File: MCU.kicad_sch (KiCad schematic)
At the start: 29 parts, among them J3 TAG-Connect, J4 BOOT, J5 USB4110-GF-A, J6 SWD, SW1 1-1571636-0, U15 12MHz, U5 RP2040, U6 W25Q16JVSSIQ

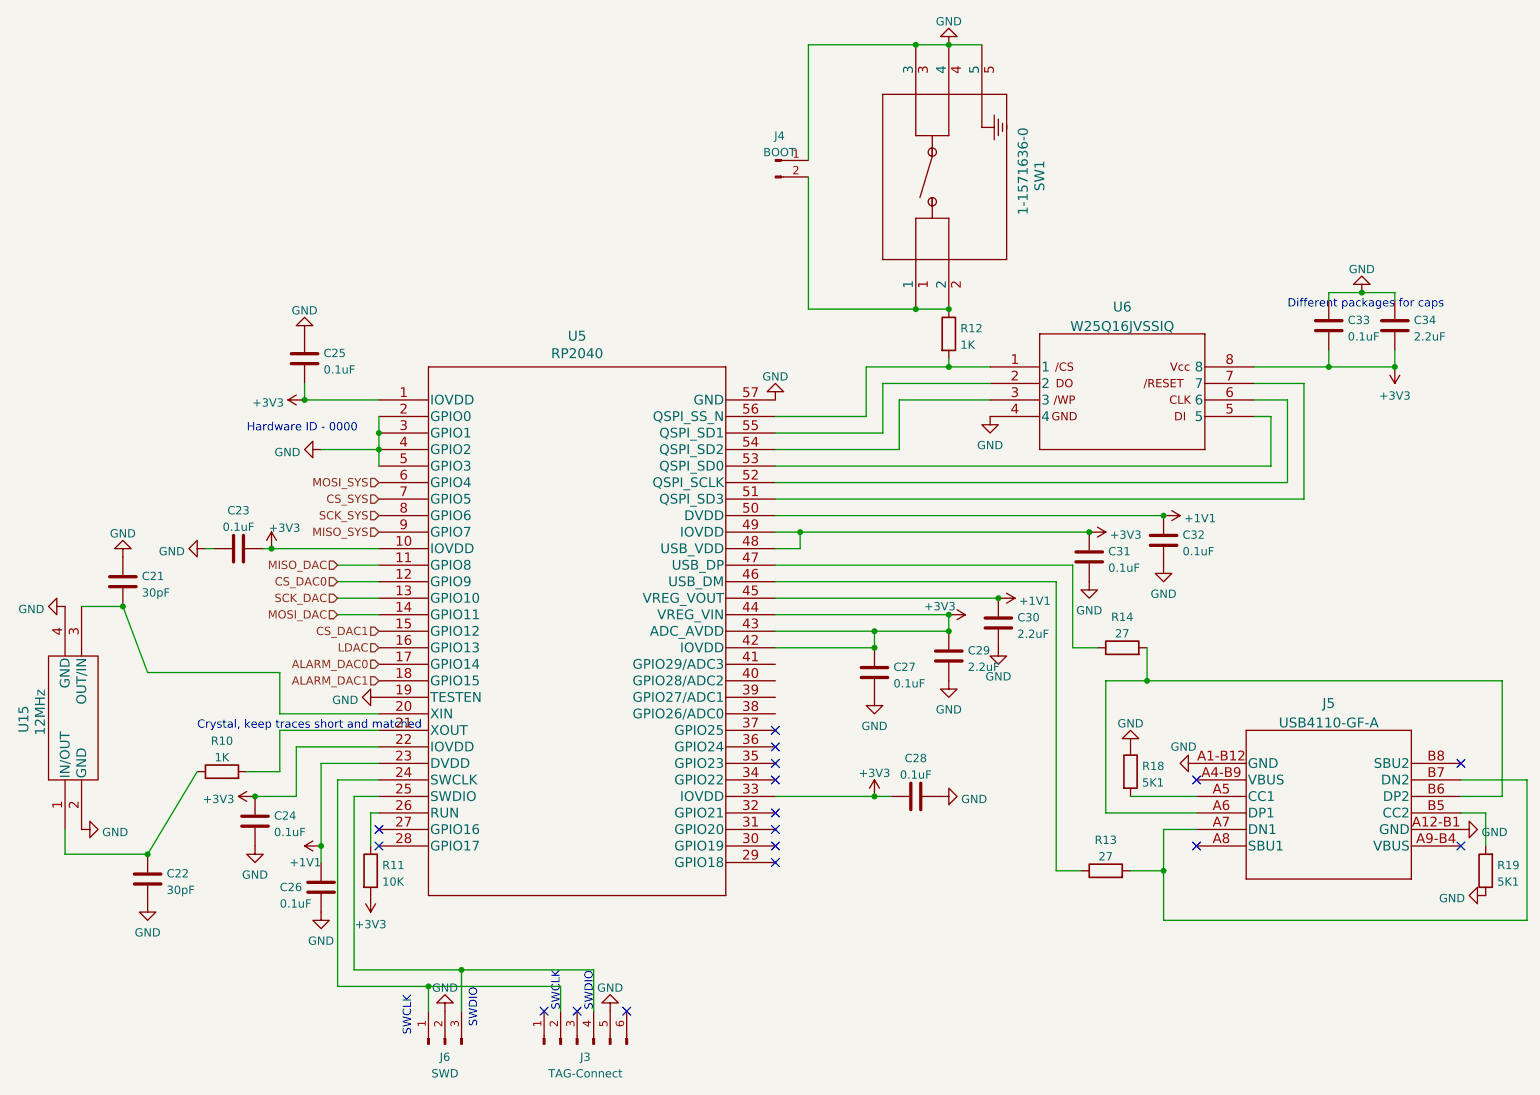
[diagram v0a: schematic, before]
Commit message: Add files via upload
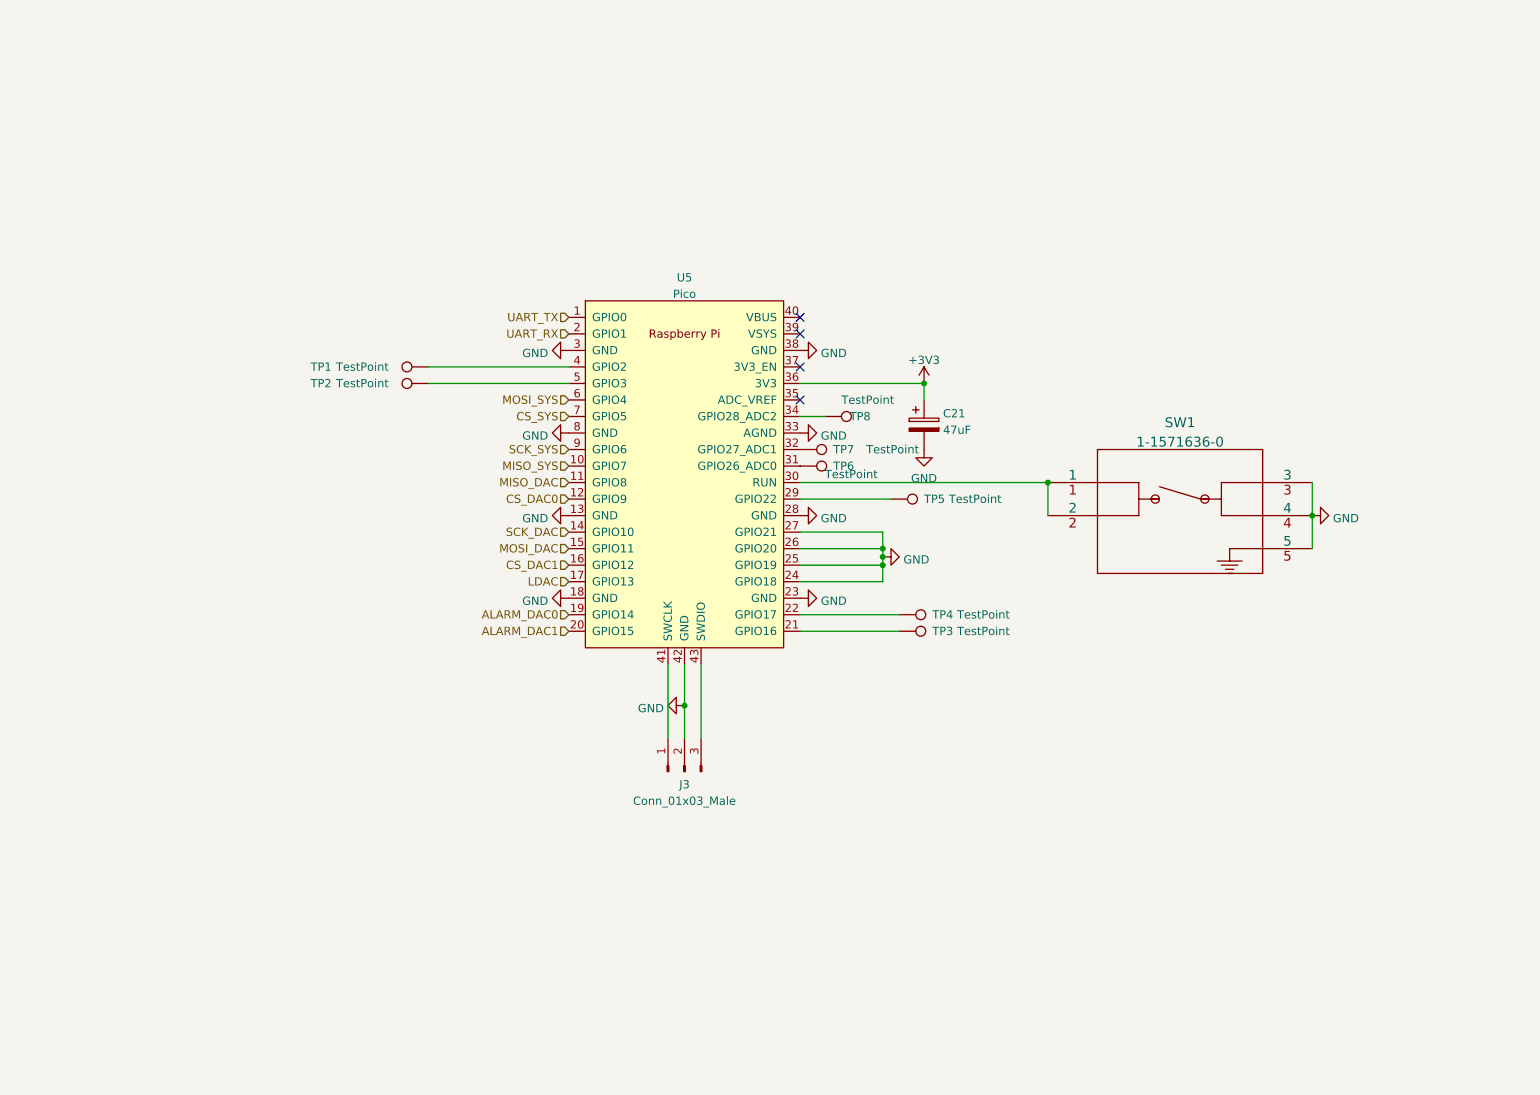
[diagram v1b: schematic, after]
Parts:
- removed C21, C22: 30pF, Capacitor_SMD:C_0402_1005Metric, symbol Device:C
- removed C23, C24, C25, C26, C27, C28, C31, C32: 0.1uF, Capacitor_SMD:C_0402_1005Metric, symbol Device:C
- removed C29, C30: 2.2uF, Capacitor_SMD:C_0603_1608Metric, symbol Device:C
- removed C33: 0.1uF, Capacitor_SMD:C_0603_1608Metric, symbol Device:C
- removed C34: 2.2uF, Capacitor_SMD:C_0805_2012Metric, symbol Device:C
- removed J3: TAG-Connect, TAG:Tag-Connect_TC2030-IDC-FP_2x03_P1.27mm_Vertical, symbol Connector:Conn_01x06_Male
- removed J4: BOOT, Connector_PinHeader_2.54mm:PinHeader_1x02_P2.54mm_Vertical, symbol Connector:Conn_01x02_Male
- removed J5: USB4110-GF-A, USB4110-GF-A:USB4110-GF-A, symbol 2022-07-06_18-10-32:USB4110-GF-A
- removed J6: SWD, Connector_PinHeader_2.54mm:PinHeader_1x03_P2.54mm_Vertical, symbol Connector:Conn_01x03_Male
- removed R10: 1K, Resistor_SMD:R_0603_1608Metric, symbol Device:R
- removed R11: 10K, Resistor_SMD:R_0402_1005Metric, symbol Device:R
- removed R12: 1K, Resistor_SMD:R_0402_1005Metric, symbol Device:R
- removed R13, R14: 27, Resistor_SMD:R_0603_1608Metric, symbol Device:R
- removed R18, R19: 5K1, Resistor_SMD:R_0603_1608Metric, symbol Device:R
- removed U15: 12MHz, ECS-120-20-33-CKM-TR:ECS-120-20-33-CKM-TR, symbol 2022-07-13_18-10-31:ECS-120-20-33-CKM-TR
- removed U5: RP2040, RP2040:RP2040, symbol 2022-06-16_17-23-33:RP2040
- removed U6: W25Q16JVSSIQ, W25Q16JVSSIQ:W25Q16JVSSIQ, symbol 2022-07-05_21-57-26:W25Q16JVSSIQ
- added C21: 47uF, Capacitor_SMD:CP_Elec_5x5.3, symbol Device:C_Polarized
- added J3: Conn_01x03_Male, Connector_PinHeader_2.54mm:PinHeader_1x03_P2.54mm_Horizontal, symbol Connector:Conn_01x03_Male
- added TP1, TP2, TP3, TP4, TP5, TP6, TP7, TP8: TestPoint, symbol Connector:TestPoint
- added U5: Pico, MCU_RaspberryPi_and_Boards:RPi_Pico_SMD_TH, symbol MCU_RaspberryPi_and_Boards:Pico
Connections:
- net +3V3: now also C21.1, U5.36 (3V3)
- net ALARM_DAC0: now also U5.19 (GPIO14)
- net ALARM_DAC1: now also U5.20 (GPIO15)
- net CS_DAC0: now also U5.12 (GPIO9)
- net CS_DAC1: now also U5.16 (GPIO12)
- net CS_SYS: now also U5.7 (GPIO5)
- net GND: now also C21.2, J3.2 (Pin_2), U5.13 (GND), U5.18 (GND), U5.23 (GND), U5.24 (GPIO18), U5.25 (GPIO19), U5.26 (GPIO20), U5.27 (GPIO21), U5.28 (GND), U5.3 (GND), U5.33 (AGND), U5.38 (GND), U5.42 (GND), U5.8 (GND)
- net LDAC: now also U5.17 (GPIO13)
- net MISO_DAC: now also U5.11 (GPIO8)
- net MISO_SYS: now also U5.10 (GPIO7)
- net MOSI_DAC: now also U5.15 (GPIO11)
- net MOSI_SYS: now also U5.6 (GPIO4)
- net SCK_DAC: now also U5.14 (GPIO10)
- net SCK_SYS: now also U5.9 (GPIO6)
- net at SW1.1, SW1.2: now also U5.30 (RUN)
- new net: TP4.1, U5.22 (GPIO17)
- new net: TP2.1, U5.5 (GPIO3)
- new net: TP7.1, U5.32 (GPIO27_ADC1)
- new net: TP8.1, U5.34 (GPIO28_ADC2)
- new net: TP6.1, U5.31 (GPIO26_ADC0)
- new net: TP3.1, U5.21 (GPIO16)
- new net: TP1.1, U5.4 (GPIO2)
- new net: J3.1 (Pin_1), U5.41 (SWCLK)
- new net: J3.3 (Pin_3), U5.43 (SWDIO)
- new net: TP5.1, U5.29 (GPIO22)
- new net UART_RX: U5.2 (GPIO1)
- new net UART_TX: U5.1 (GPIO0)
- no-connect marks 17 -> 4
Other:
- note removed: "Crystal, keep traces short and matched"
- note removed: "Different packages for caps"
- note removed: "Hardware ID - 0000"
- note removed: "SWCLK"
- note removed: "SWDIO"

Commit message: Add files via upload
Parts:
- TP1, TP2, TP3, TP4, TP5, TP6, TP7, TP8: footprint (none) -> TestPoint:TestPoint_Bridge_Pitch2.0mm_Drill0.7mm
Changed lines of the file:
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@@
       (effects (font (size 1.27 1.27)) (justify left))
     )
-    (property "Footprint" "" (id 2) (at 158.75 114.3 0)
+    (property "Footprint" "TestPoint:TestPoint_Bridge_Pitch2.0mm_Drill0.7mm" (id 2) (at 158.75 114.3 0)
       (effects (font (size 1.27 1.27)) hide)
     )
@@
     (property "Reference" "TP2" (id 0) (at 69.85 73.66 90))
     (property "Value" "TestPoint" (id 1) (at 76.2 73.66 90))
-    (property "Footprint" "" (id 2) (at 86.36 68.58 0)
+    (property "Footprint" "TestPoint:TestPoint_Bridge_Pitch2.0mm_Drill0.7mm" (id 2) (at 86.36 68.58 0)
       (effects (font (size 1.27 1.27)) hide)
     )
@@
       (effects (font (size 1.27 1.27)) (justify left))
     )
-    (property "Footprint" "" (id 2) (at 143.51 88.9 0)
+    (property "Footprint" "TestPoint:TestPoint_Bridge_Pitch2.0mm_Drill0.7mm" (id 2) (at 143.51 88.9 0)
       (effects (font (size 1.27 1.27)) hide)
     )
@@
       (effects (font (size 1.27 1.27)) (justify left))
     )
-    (property "Footprint" "" (id 2) (at 147.32 83.82 0)
+    (property "Footprint" "TestPoint:TestPoint_Bridge_Pitch2.0mm_Drill0.7mm" (id 2) (at 147.32 83.82 0)
       (effects (font (size 1.27 1.27)) hide)
     )
@@
       (effects (font (size 1.27 1.27)) (justify left))
     )
-    (property "Footprint" "" (id 2) (at 143.51 91.44 0)
+    (property "Footprint" "TestPoint:TestPoint_Bridge_Pitch2.0mm_Drill0.7mm" (id 2) (at 143.51 91.44 0)
       (effects (font (size 1.27 1.27)) hide)
     )
@@
       (effects (font (size 1.27 1.27)) (justify left))
     )
-    (property "Footprint" "" (id 2) (at 158.75 116.84 0)
+    (property "Footprint" "TestPoint:TestPoint_Bridge_Pitch2.0mm_Drill0.7mm" (id 2) (at 158.75 116.84 0)
       (effects (font (size 1.27 1.27)) hide)
     )
@@
     (property "Reference" "TP1" (id 0) (at 69.85 71.12 90))
     (property "Value" "TestPoint" (id 1) (at 76.2 71.12 90))
-    (property "Footprint" "" (id 2) (at 86.36 66.04 0)
+    (property "Footprint" "TestPoint:TestPoint_Bridge_Pitch2.0mm_Drill0.7mm" (id 2) (at 86.36 66.04 0)
       (effects (font (size 1.27 1.27)) hide)
     )
@@
       (effects (font (size 1.27 1.27)) (justify left))
     )
-    (property "Footprint" "" (id 2) (at 157.48 96.52 0)
+    (property "Footprint" "TestPoint:TestPoint_Bridge_Pitch2.0mm_Drill0.7mm" (id 2) (at 157.48 96.52 0)
       (effects (font (size 1.27 1.27)) hide)
     )
@@
   (symbol (lib_id "power:+3V3") (at 162.56 73.66 0) (unit 1)
     (in_bom yes) (on_board yes) (fields_autoplaced)
-    (property "Reference" "#PWR?" (id 0) (at 162.56 77.47 0)
-      (effects (font (size 1.27 1.27)) hide)
-    )
+    (property "Reference" "#PWR0102" (id 0) (at 162.56 77.47 0)
+      (effects (font (size 1.27 1.27)) hide)
+    )
